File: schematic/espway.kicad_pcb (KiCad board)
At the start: 2 copper layers, 35 parts, among them J1 CONN_01X02, J2 CONN_01X02, J3 CONN_01X04_MALE, SW1 SW_Push, U1 LM1117-3.3, U2 ESP-12E, U3 DRV8835, U4 LSM6DS3

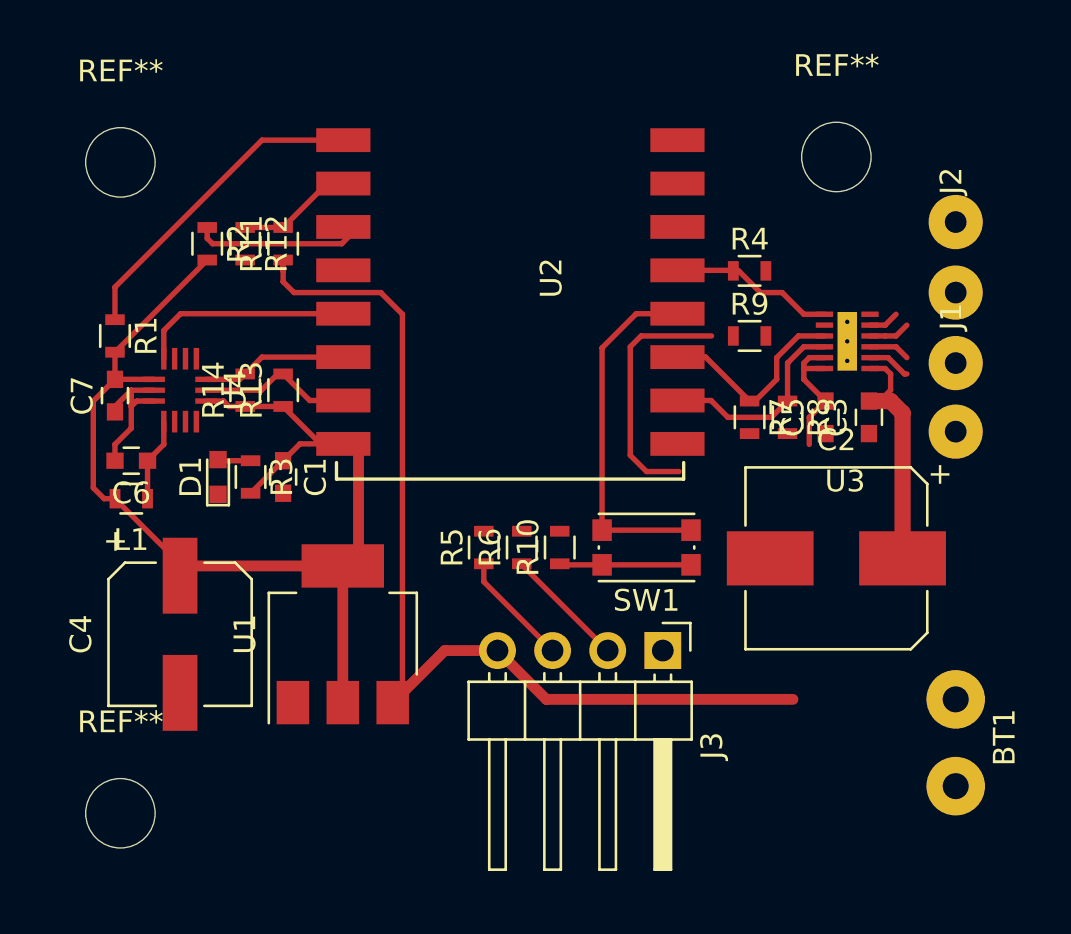
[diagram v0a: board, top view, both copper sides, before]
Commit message: Committing before rerouting
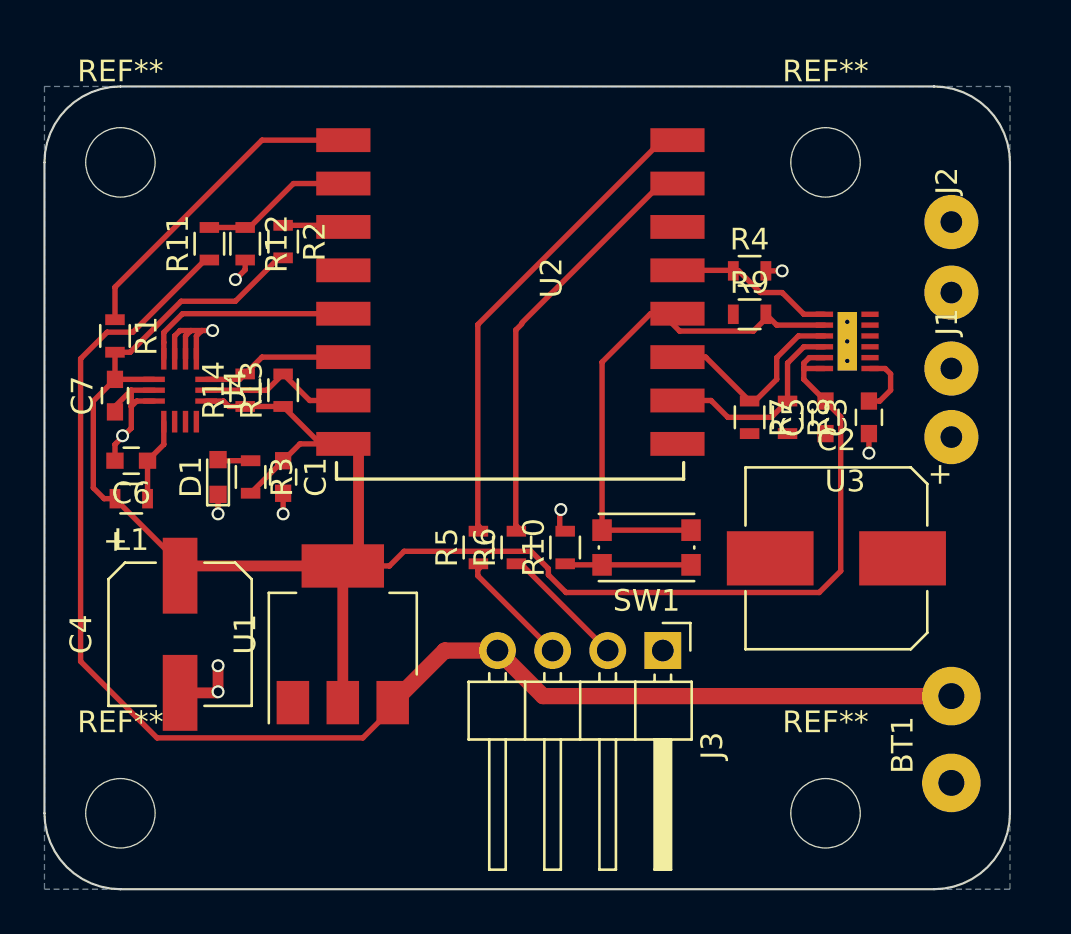
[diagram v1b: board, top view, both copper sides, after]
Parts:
- added REF**: MountingHole_3.2mm_M3, Mounting_Holes:MountingHole_3.2mm_M3, F.Cu at (162.0, 154.0)
- moved BT1 4.15 mm to (167.8, 148.6), turned to 270 degrees
- moved R2 3.50 mm to (137.0, 127.7)
- moved R11 3.40 mm to (133.6, 127.8)
- moved R9 1.00 mm to (158.5, 131.0)
- moved REF** 0.56 mm to (162.0, 124.0)
- moved J1 0.32 mm to (167.8, 126.5)
- moved R10 0.25 mm to (150.0, 141.8)
- moved R5 0.25 mm to (146.0, 141.8)
- moved R6 0.25 mm to (147.8, 141.8)
- moved J2 0.20 mm to (167.8, 120.0)
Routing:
- net +3V3: track 60.6 -> 94.6 mm
- net Net-(R5-Pad2): track 0.00 -> 21.7 mm
- net Net-(R6-Pad2): track 0.00 -> 18.9 mm
- net GND: track 7.07 -> 21.4 mm, vias 0 -> 10
- net +BATT: track 57.6 -> 69.7 mm
- net (no net): track 11.5 -> 0.00 mm
- net BPHASE: track 19.2 -> 28.3 mm
- net Net-(R2-Pad1): track 7.90 -> 3.21 mm
- net ADC: track 6.06 -> 9.16 mm
- net Net-(J1-Pad2): track 2.01 -> 0.00 mm
- net Net-(J2-Pad2): track 1.91 -> 0.00 mm
- net Net-(J1-Pad1): track 1.91 -> 0.00 mm
- net Net-(J2-Pad1): track 1.41 -> 0.00 mm
- added copper zone on B.Cu, net GND
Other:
- board outline added: 44.5 x 37 mm
